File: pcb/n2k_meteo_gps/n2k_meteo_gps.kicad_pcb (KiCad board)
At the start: 2 copper layers, 45.5 x 50.5 mm, 24 parts, among them J1 I2C, J10 3.3-5V, J2 1W_DHT22, J3 VE.Direct, J4 I2C_BME280, J5 5V switch, J6 GPS, J7 I2C, J8 CAN Term, J9 N2K, U2 TSR_1-2450, U3 MCP2562-E-P, U4 PC817, U5 ESP32-C3_SUPERMINI

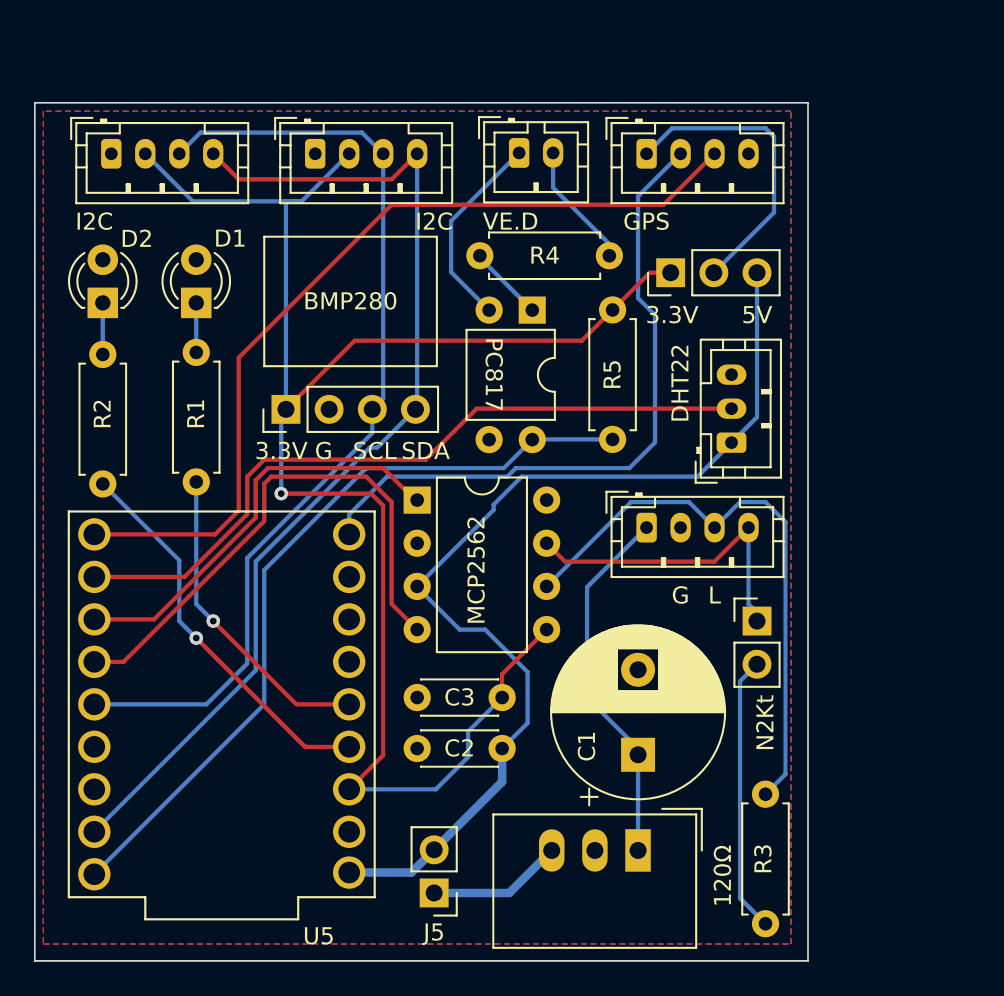
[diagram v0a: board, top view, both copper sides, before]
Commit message: pcb
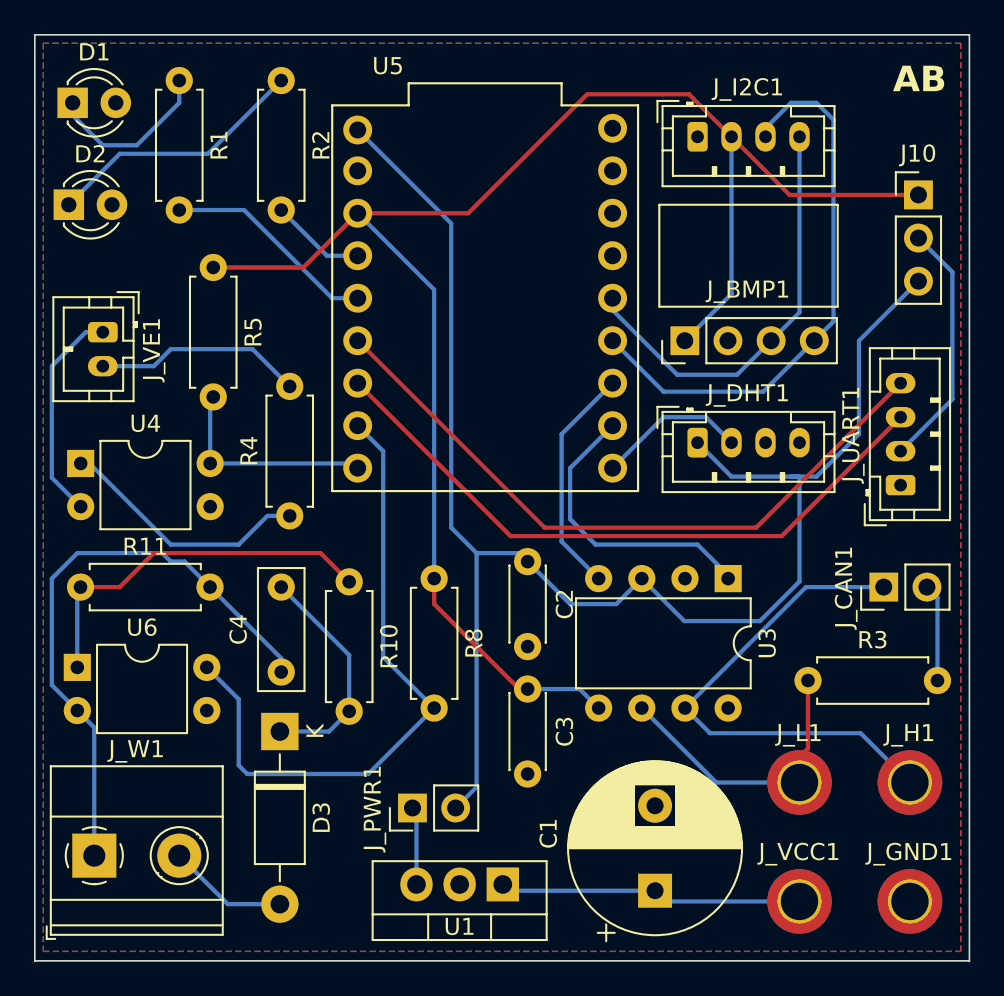
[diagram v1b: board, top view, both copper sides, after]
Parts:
- removed J1, J7: I2C, Connector_JST:JST_PH_B4B-PH-K_1x04_P2.00mm_Vertical
- removed J2: 1W_DHT22, Connector_JST:JST_PH_B3B-PH-K_1x03_P2.00mm_Vertical
- removed J3: VE.Direct, Connector_JST:JST_PH_B2B-PH-K_1x02_P2.00mm_Vertical
- removed J4: I2C_BME280, Connector_PinHeader_2.54mm:PinHeader_1x04_P2.54mm_Vertical
- removed J5: 5V switch, Connector_PinHeader_2.54mm:PinHeader_1x02_P2.54mm_Vertical
- removed J6: GPS, Connector_JST:JST_PH_B4B-PH-K_1x04_P2.00mm_Vertical
- removed J8: CAN Term, Connector_PinHeader_2.54mm:PinHeader_1x02_P2.54mm_Vertical
- removed J9: N2K, Connector_JST:JST_PH_B4B-PH-K_1x04_P2.00mm_Vertical
- removed U2: TSR_1-2450, Converter_DCDC:Converter_DCDC_TRACO_TSR-1_THT
- added C4: 10nanoF, Capacitor_THT:C_Disc_D7.0mm_W2.5mm_P5.00mm, F.Cu at (33.5, 78.2)
- added D3: 1N4001, Diode_THT:D_DO-41_SOD81_P10.16mm_Horizontal, F.Cu at (33.5, 81.8)
- added J_BMP1: I2C_BME280, Connector_PinHeader_2.54mm:PinHeader_1x04_P2.54mm_Vertical, F.Cu at (57.3, 58.8)
- added J_CAN1: CAN Term, Connector_PinHeader_2.54mm:PinHeader_1x02_P2.54mm_Vertical, F.Cu at (69.0, 73.2)
- added J_DHT1: 1W_DHT22, Connector_JST:JST_PH_B4B-PH-K_1x04_P2.00mm_Vertical, F.Cu at (58.0, 64.8)
- added J_GND1: CAN GND, MountingHole:MountingHole_2.2mm_M2_DIN965_Pad_TopBottom, F.Cu at (70.5, 91.8)
- added J_H1: CAN H, MountingHole:MountingHole_2.2mm_M2_DIN965_Pad_TopBottom, F.Cu at (70.5, 84.8)
- added J_I2C1: I2C, Connector_JST:JST_PH_B4B-PH-K_1x04_P2.00mm_Vertical, F.Cu at (58.0, 46.8)
- added J_L1: CAN L, MountingHole:MountingHole_2.2mm_M2_DIN965_Pad_TopBottom, F.Cu at (64.0, 84.8)
- added J_PWR1: 5V switch, Connector_PinHeader_2.54mm:PinHeader_1x02_P2.54mm_Vertical, F.Cu at (41.3, 86.2)
- added J_UART1: GPS, Connector_JST:JST_PH_B4B-PH-K_1x04_P2.00mm_Vertical, F.Cu at (70.0, 67.2)
- added J_VCC1: CAN 12V, MountingHole:MountingHole_2.2mm_M2_DIN965_Pad_TopBottom, F.Cu at (64.0, 91.8)
- added J_VE1: VE.Direct, Connector_JST:JST_PH_B2B-PH-K_1x02_P2.00mm_Vertical, F.Cu at (23.1, 58.2)
- added J_W1: Engine RPM Input, TerminalBlock_Phoenix:TerminalBlock_Phoenix_MKDS-1,5-2_1x02_P5.00mm_Horizontal, F.Cu at (22.6, 89.1)
- added R10: 10K, Resistor_THT:R_Axial_DIN0207_L6.3mm_D2.5mm_P7.62mm_Horizontal, F.Cu at (37.5, 72.9)
- added R11: 4.7K, Resistor_THT:R_Axial_DIN0207_L6.3mm_D2.5mm_P7.62mm_Horizontal, F.Cu at (21.7, 73.2)
- added R8: 4.7K, Resistor_THT:R_Axial_DIN0207_L6.3mm_D2.5mm_P7.62mm_Horizontal, F.Cu at (42.5, 72.8)
- added U1: LM7805_TO220, Package_TO_SOT_THT:TO-220-3_Vertical, F.Cu at (46.6, 90.8)
- added U6: PC817, Package_DIP:DIP-4_W7.62mm, F.Cu at (21.6, 78.0)
- C1: value C_470microF -> 100uF
- C2, C3: value 10nanoF -> 100nF
- U5: footprint esp32_c3_supermini:WAVESHARE_DEVKIT_ESP32-C3-ZERO -> Library:WAVESHARE_DEVKIT_ESP32-C3-ZERO
- moved U5 28.5 mm to (45.5, 56.2), turned to 0 degrees
- moved U4 28.1 mm to (21.8, 66.0), turned to 0 degrees
- moved R5 23.6 mm to (29.6, 54.4)
- moved R2 19.2 mm to (33.5, 43.4)
- moved R4 19.0 mm to (34.0, 69.1), turned to 90 degrees
- moved U3 18.9 mm to (59.9, 72.8), turned to -90 degrees
- moved R1 16.0 mm to (27.6, 43.4)
- moved J10 15.3 mm to (71.0, 50.2), turned to 0 degrees
- moved D1 13.8 mm to (21.3, 44.8), turned to 0 degrees
- moved C2 11.1 mm to (48.0, 71.8), turned to -90 degrees
- moved C1 8.06 mm to (55.5, 91.1)
- moved R3 7.14 mm to (64.5, 78.8), turned to 0 degrees
- moved D2 6.11 mm to (21.1, 50.8), turned to 0 degrees
- moved C3 1.58 mm to (48.0, 79.2), turned to -90 degrees
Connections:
- R5 pad 2: Net-(U5-GPIO21) -> Net-(U5-GPIO5)
- U4 pad 4: Net-(U5-GPIO21) -> Net-(U5-GPIO5)
- U5 pad 2: unconnected-(U5-GPIO2-Pad2) -> Net-(J_UART1-Pin_4)
- U5 pad 20: Net-(J1-Pin_4) -> unconnected-(U5-GPIO20-Pad20)
- U5 pad 21: Net-(U5-GPIO21) -> unconnected-(U5-GPIO21-Pad21)
- U5 pad 3: unconnected-(U5-GPIO3-Pad3) -> Net-(J_UART1-Pin_3)
- U5 pad 4: unconnected-(U5-GPIO4-Pad4) -> Net-(U5-GPIO4)
- U5 pad 5: Net-(J6-Pin_2) -> Net-(U5-GPIO5)
- U5 pad 7: Net-(J2-Pin_2) -> Net-(U3-TXD)
- U5 pad 8: Net-(U3-TXD) -> Net-(U3-RXD)
- U5 pad 9: Net-(U3-RXD) -> Net-(J_BMP1-Pin_4)
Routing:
- net Net-(J1-Pin_4): track 61.3 -> 0.00 mm
- net Net-(U5-GPIO21): track 45.7 -> 0.00 mm
- net Net-(J2-Pin_2): track 42.9 -> 0.00 mm
- net Net-(J_DHT1-Pin_2): track 51.1 -> 8.86 mm
- net Net-(J_UART1-Pin_4): track 0.00 -> 40.0 mm
- net Net-(J6-Pin_2): track 39.4 -> 0.00 mm
- net Net-(J_UART1-Pin_3): track 0.00 -> 38.6 mm
- net Net-(U5-GPIO4): track 0.00 -> 38.4 mm
- net +5V: track 59.7 -> 94.7 mm
- net Net-(J_W1-Pin_1): track 0.00 -> 34.8 mm
- net Net-(J_BMP1-Pin_4): track 0.00 -> 33.4 mm
- net Net-(J_BMP1-Pin_3): track 56.3 -> 25.1 mm
- net Net-(R10-Pad1): track 0.00 -> 22.1 mm
- net Net-(U3-RXD): track 32.1 -> 13.6 mm
- net Net-(U5-GPIO0): track 23.0 -> 5.61 mm, vias 1 -> 0
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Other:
- board size 45.5 x 50.5 mm -> 55 x 54.5 mm
- board text added: "AB"
- board text removed: "120Ω"
- board text removed: "3.3V"
- board text removed: "5V"
- board text removed: "BMP280"
- board text removed: "DHT22"
- board text removed: "G"
- board text removed: "GPS"
- board text removed: "I2C"
- board text removed: "L"
- board text removed: "MCP2562"
- board text removed: "N2Kt"
- board text removed: "PC817"
- board text removed: "SCL"
- board text removed: "SDA"
- board text removed: "VE.D"
